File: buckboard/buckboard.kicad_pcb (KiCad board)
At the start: 2 copper layers, 163.5 x 65.4 mm, 29 parts

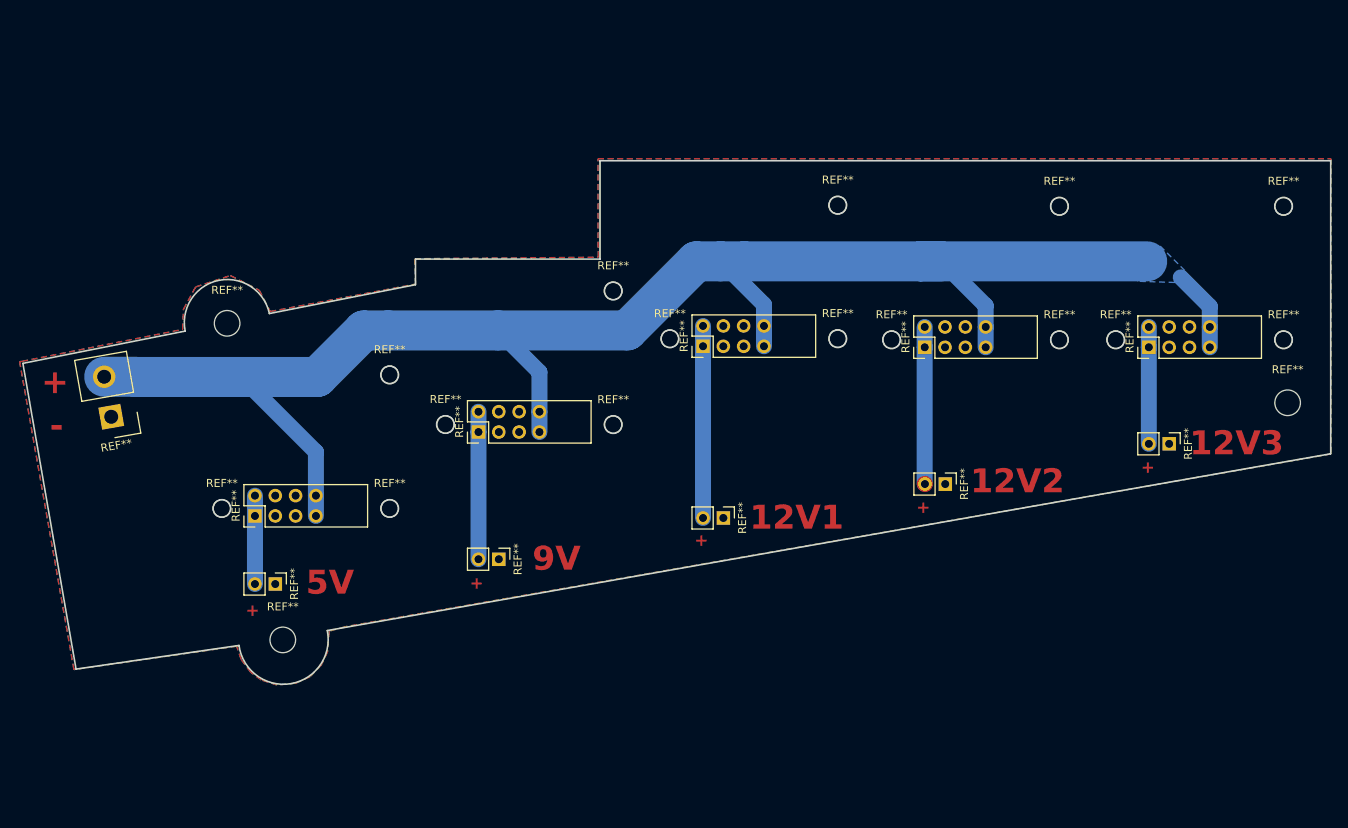
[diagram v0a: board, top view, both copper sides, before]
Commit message: V1.2
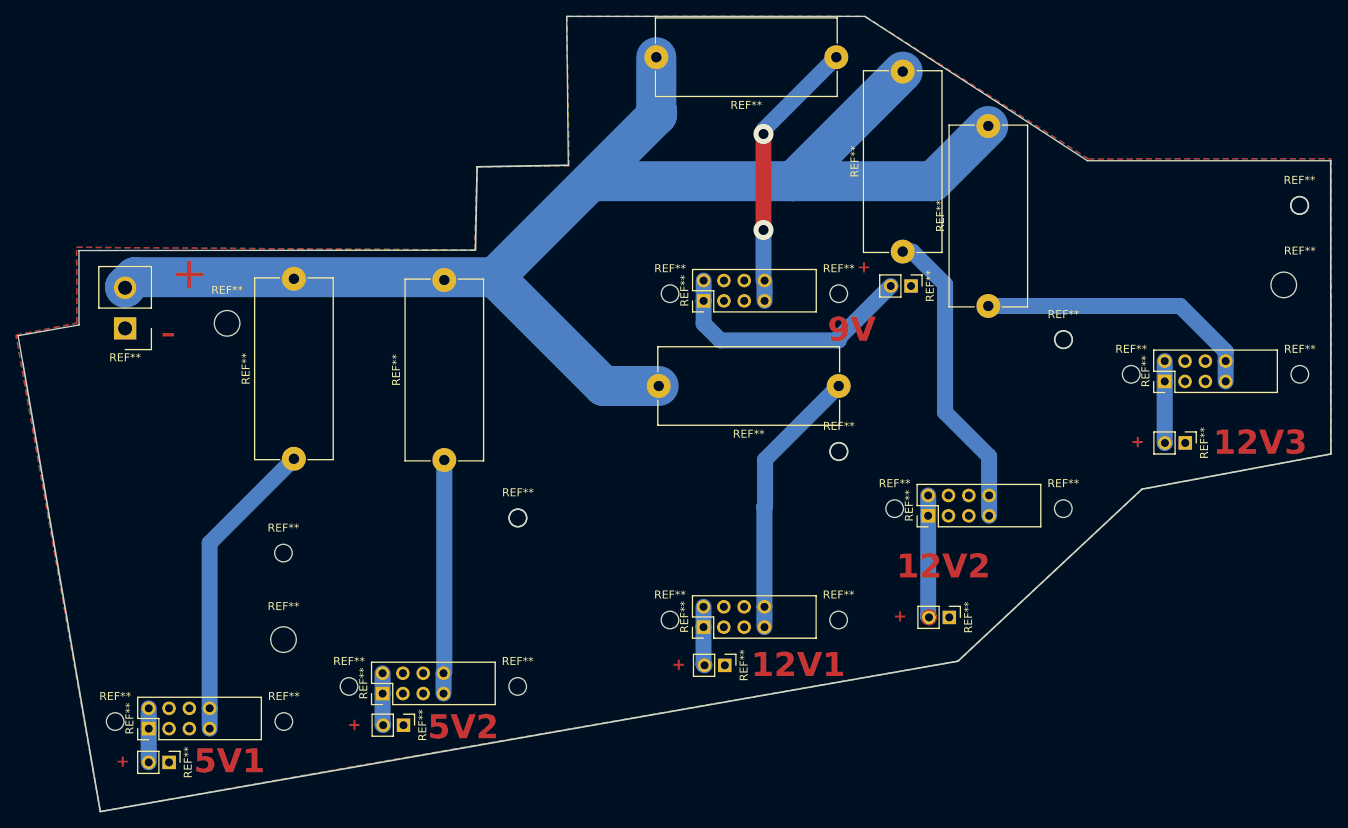
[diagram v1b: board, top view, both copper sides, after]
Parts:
- removed the REF** at (146.8, 66.7)
- added REF**: Fuseholder_Cylinder-5x20mm_Schurter_0031_8201_Horizontal_Op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, Fuse:Fuseholder_Cylinder-5x20mm_Schurter_0031_8201_Horizontal_Open, F.Cu at (125.7, 87.8)
- added REF**: Fuseholder_Cylinder-5x20mm_Schurter_0031_8201_Horizontal_Op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, Fuse:Fuseholder_Cylinder-5x20mm_Schurter_0031_8201_Horizontal_Open, F.Cu at (106.9, 87.7)
- added REF**: Fuseholder_Cylinder-5x20mm_Schurter_0031_8201_Horizontal_Op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, Fuse:Fuseholder_Cylinder-5x20mm_Schurter_0031_8201_Horizontal_Open, F.Cu at (175.0, 78.6)
- added REF**: PinHeader_2x06_P2.54mm_Vertical, Connector_PinHeader_2.54mm:PinHeader_2x06_P2.54mm_Vertical, F.Cu at (158.1, 108.7)
- added REF**: PinHeader_1x02_P2.54mm_Vertical, Connector_PinHeader_2.54mm:PinHeader_1x02_P2.54mm_Vertical, F.Cu at (160.8, 113.5)
- added REF**: MountingHole_2.2mm_M2, MountingHole:MountingHole_2.2mm_M2, F.Cu at (175.0, 107.9)
- added REF**: Fuseholder_Cylinder-5x20mm_Schurter_0031_8201_Horizontal_Op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, Fuse:Fuseholder_Cylinder-5x20mm_Schurter_0031_8201_Horizontal_Open, F.Cu at (174.7, 37.5)
- added REF**: MountingHole_2.2mm_M2, MountingHole:MountingHole_2.2mm_M2, F.Cu at (153.9, 107.9)
- added REF**: Fuseholder_Cylinder-5x20mm_Schurter_0031_8201_Horizontal_Op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, Fuse:Fuseholder_Cylinder-5x20mm_Schurter_0031_8201_Horizontal_Open, F.Cu at (193.7, 68.6)
- added REF**: Fuseholder_Cylinder-5x20mm_Schurter_0031_8201_Horizontal_Op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, Fuse:Fuseholder_Cylinder-5x20mm_Schurter_0031_8201_Horizontal_Open, F.Cu at (183.0, 61.8)
- added REF**: MountingHole_2.2mm_M2, MountingHole:MountingHole_2.2mm_M2, F.Cu at (175.0, 86.8)
- moved REF** 61.8 mm to (184.0, 66.1)
- moved REF** 59.1 mm to (113.8, 116.2)
- moved REF** 59.1 mm to (134.9, 116.2)
- moved REF** 59.1 mm to (118.0, 117.0)
- moved REF** 55.9 mm to (134.9, 95.1)
- moved REF** 47.6 mm to (120.6, 121.0)
- moved REF** 32.6 mm to (175.0, 67.1)
- moved REF** 32.6 mm to (158.1, 68.0)
- moved REF** 32.5 mm to (153.9, 67.1)
- moved REF** 29.8 mm to (84.6, 120.5)
- moved REF** 29.7 mm to (105.6, 120.5)
- moved REF** 29.7 mm to (88.8, 121.4)
- moved REF** 26.0 mm to (91.3, 125.6)
- moved REF** 26.0 mm to (105.6, 99.5)
- moved REF** 21.1 mm to (203.1, 93.9)
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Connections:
- net 12V1 renamed 5V2
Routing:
- net VIN: track 211.2 -> 389.3 mm, vias 0 -> 2
- net 5V2: track 24.0 -> 6.53 mm
- net 9V: track 18.4 -> 32.6 mm
- net 12V1: track 0.00 -> 7.37 mm
- net 12V3: track 14.6 -> 10.2 mm
- net 12V2: track 19.6 -> 15.3 mm
- net 5V: track 11.0 -> 6.76 mm
- removed copper zone on B.Cu, net VIN
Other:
- board size 163.5 x 65.4 mm -> 164.1 x 99.4 mm
- board text added: "5V1"
- board text added: "5V2"
- board text removed: "5V"
